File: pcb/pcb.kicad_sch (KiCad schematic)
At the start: 36 parts, among them J1 Ribbon Cable Header, J2 Ribbon Cable Header, J3 UPDI, SW1 MX Grey w/ LED, SW2 MX Grey w/ LED, SW3 1241.1100.7095, SW4 SW_SPST, U1 Display Driver, U2 Display Driver, U3 MCU, U4 OR, 2 Channels, U5 5V Buck Voltage Regulator, Y1 32.768 kHz

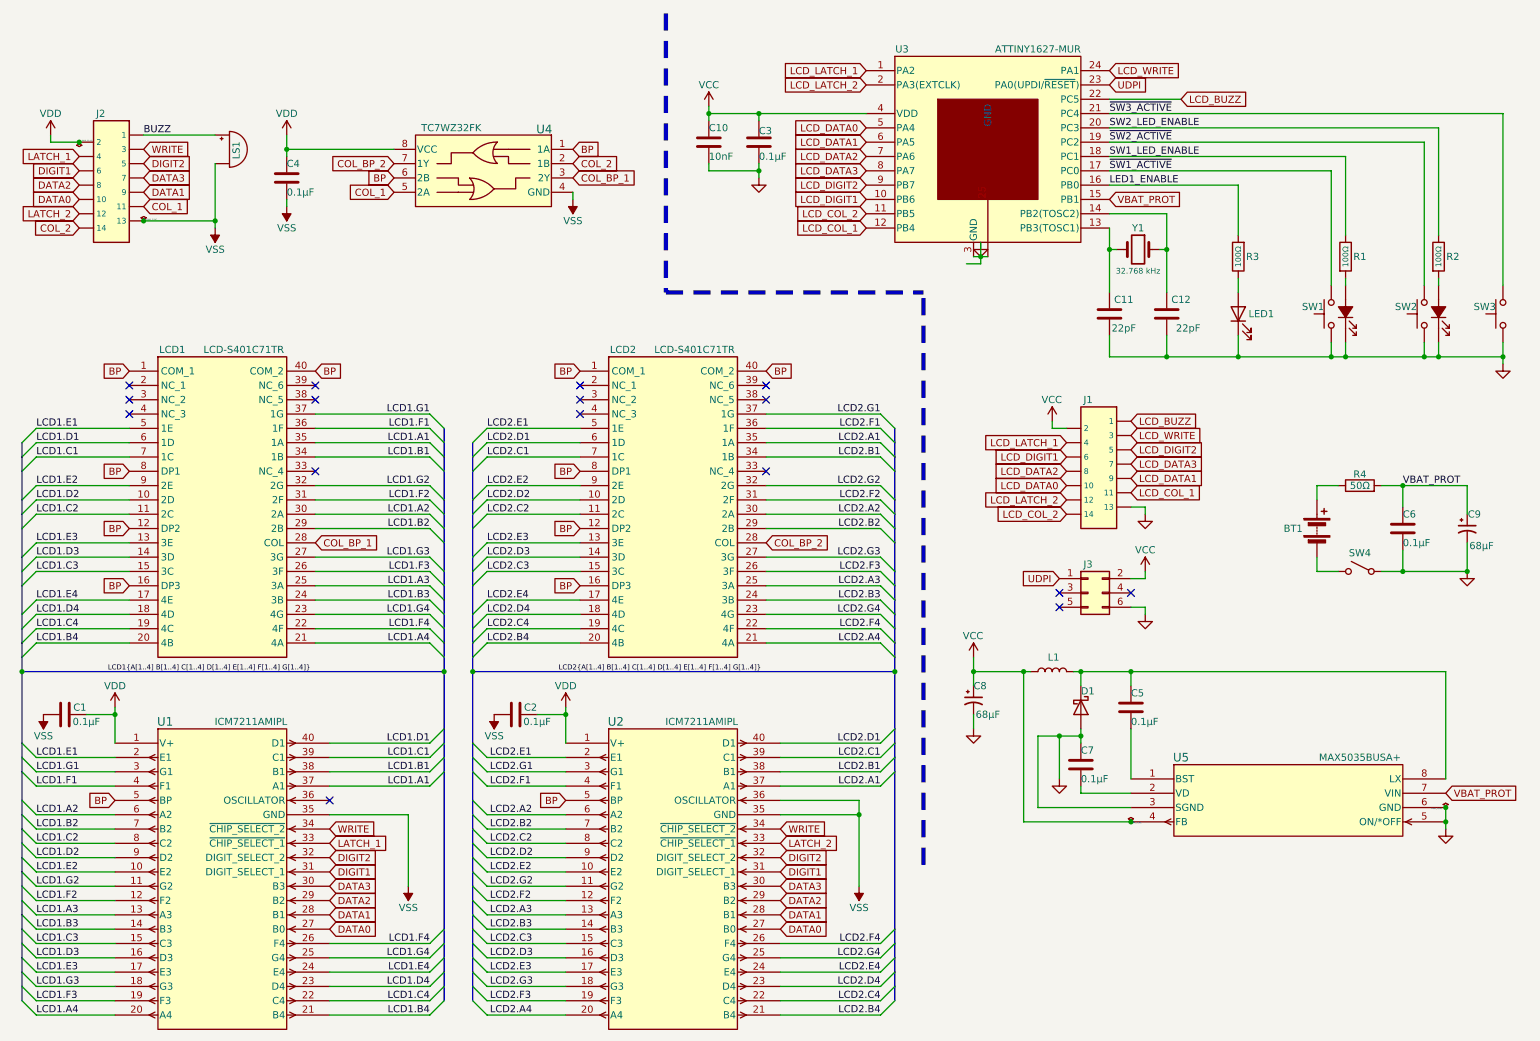
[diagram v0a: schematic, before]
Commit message: 0.2.0
Signed-off-by: Michael Darr <michael.e.darr@gmail.com>
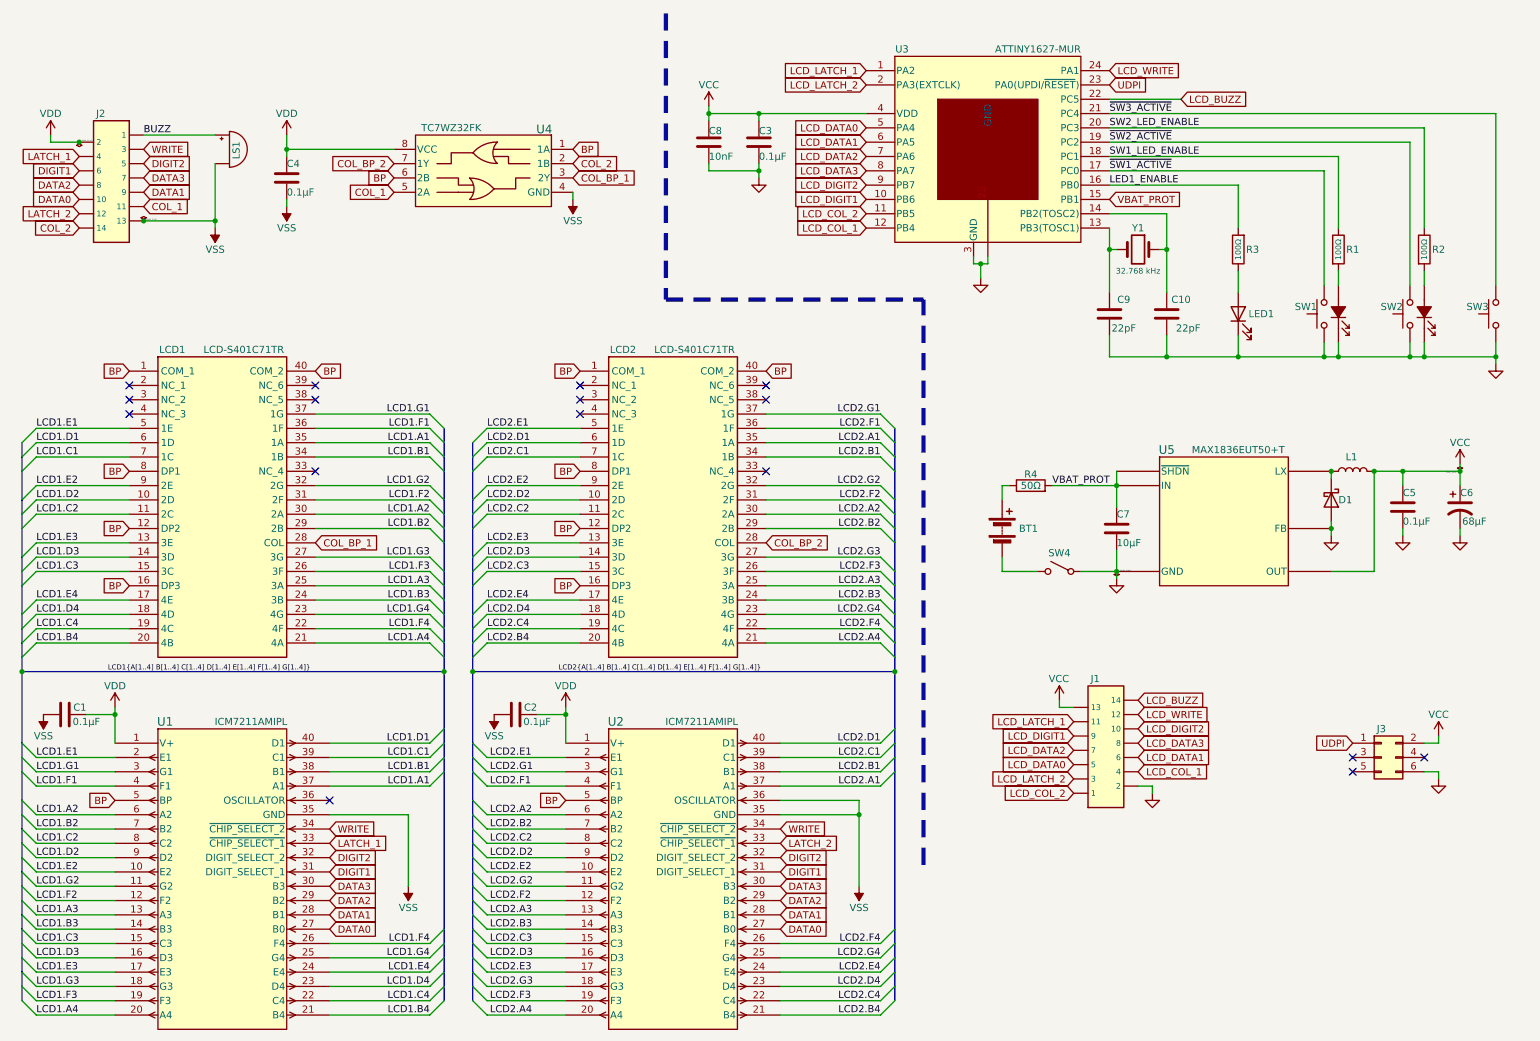
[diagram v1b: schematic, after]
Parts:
- removed C5: 0.1µF, Capacitor_SMD:C_0805_2012Metric_Pad1.18x1.45mm_HandSolder, symbol Device:C
- removed C9: 68µF, chess_clock:TPSD686K010R0100, symbol Device:C_Polarized_Small_US
- removed U5: 5V Buck Voltage Regulator, chess_clock:MAX5035BUSA+, symbol Clock-Parts:MAX5035BUSA+
- added U5: Voltage Regulator, chess_clock:MAX1836EUT50+T, symbol Clock-Parts:MAX1836EUT50+T
- BT1: footprint Connector_Wire:SolderWire-0.15sqmm_1x02_P4mm_D0.5mm_OD1.5mm -> chess_clock:BATTERY
- C6: renamed from C8; symbol Device:C_Polarized_Small_US -> Device:C_Polarized_US
- C7: value 0.1µF -> 10µF; PN CL21B104KBCNNNC -> CL21A106KOQNNNE
- C8: renamed from C10; PN (none) -> CL21B103KBANNNC
- renumbered C12 to C10, C6 to C5, C11 to C9
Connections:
- net GND: now also C7.2, J1.2, U5.1 (FB), U5.2 (GND); no longer C7.1, J1.13
- net LCD_BUZZ: now also J1.14; no longer J1.1
- net LCD_COL_1: now also J1.4; no longer J1.11
- net LCD_COL_2: now also J1.1; no longer J1.14
- net LCD_DATA0: now also J1.5; no longer J1.10
- net LCD_DATA1: now also J1.6; no longer J1.9
- net LCD_DATA2: now also J1.7; no longer J1.8
- net LCD_DATA3: now also J1.8; no longer J1.7
- net LCD_DIGIT1: now also J1.9; no longer J1.6
- net LCD_DIGIT2: now also J1.10; no longer J1.5
- net LCD_LATCH_1: now also J1.11; no longer J1.4
- net LCD_LATCH_2: now also J1.3; no longer J1.12
- net LCD_WRITE: now also J1.12; no longer J1.3
- net VBAT_PROT: now also C7.1, U5.3 (IN), U5.5 (~{SHDN}); no longer C5.1
- net VCC: now also C5.1, J1.13, U5.6 (OUT); no longer J1.2
- net at D1.1 (K), L1.2: now also U5.4 (LX)
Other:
- moved on the sheet: BT1, C5, C6, D1, J1, J3, L1, R1, R2, R3, R4, SW1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
